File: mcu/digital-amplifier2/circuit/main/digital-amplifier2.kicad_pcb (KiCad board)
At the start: 2 copper layers, 100 x 100 mm, 173 parts, among them J1 USB_B, J2 Barrel_Jack_Switch, J3 AudioJack3_Switch, J4 AudioJack4, J5 ec11, J6 ext_sai, J7 swd, Q1 s8550, SW1 sw1, SW2 sw2, SW3 sw3, T1 Transformer_diy_01, U1 STM32F446RETx, U10 LP2992AIM5-5.0_NOPB, U11 LP2992AIM5-3.3_NOPB, U12 PCM1792A, U13 OPA4134, U2 LP2992AIM5-3.3_NOPB, U3 TPS55340, U4 LP2992AIM5-3.3_NOPB, U5 DLT11H0, U6 SJR-BTM331, U7 TPA6120A2, U8 LT3045xMSE-1, U9 LT3094xMSE, Y1 5032 8m

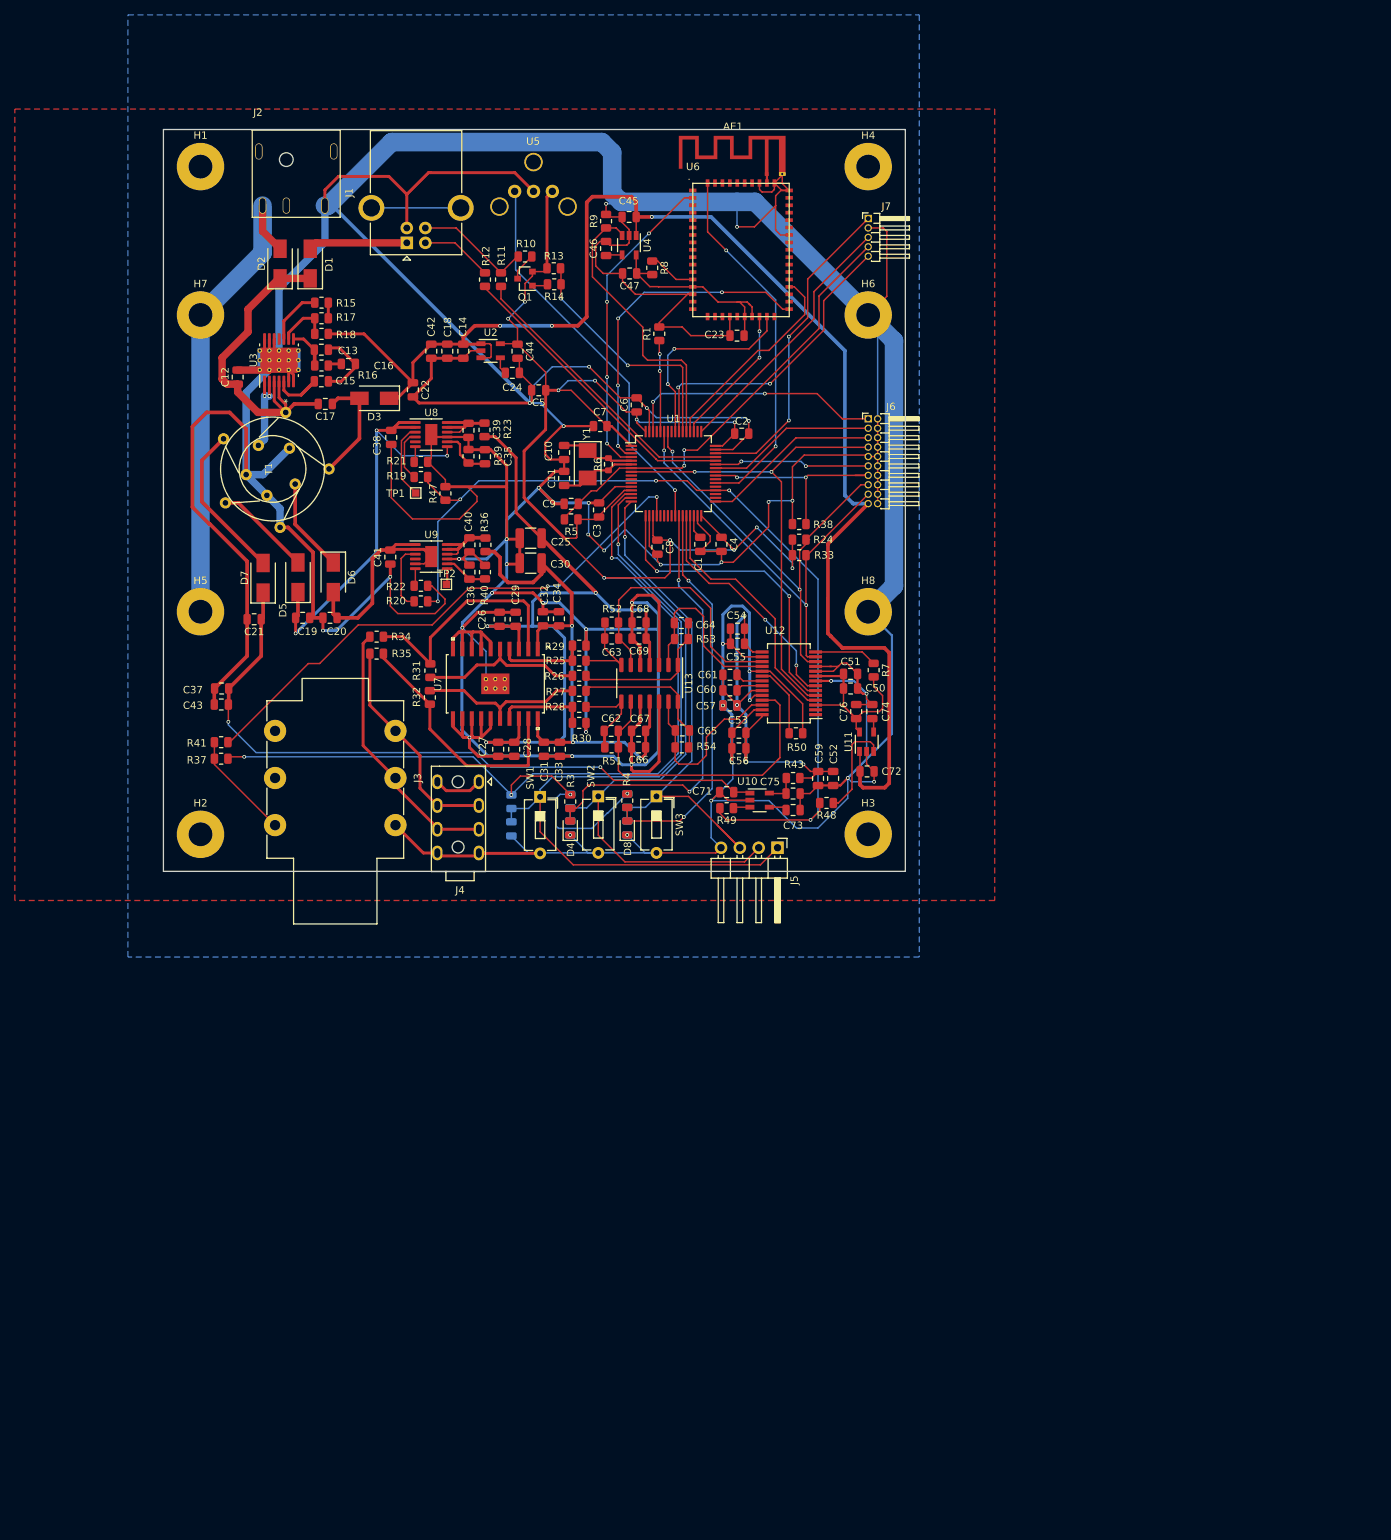
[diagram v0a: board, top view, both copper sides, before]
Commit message: digital-amplifier2_v8
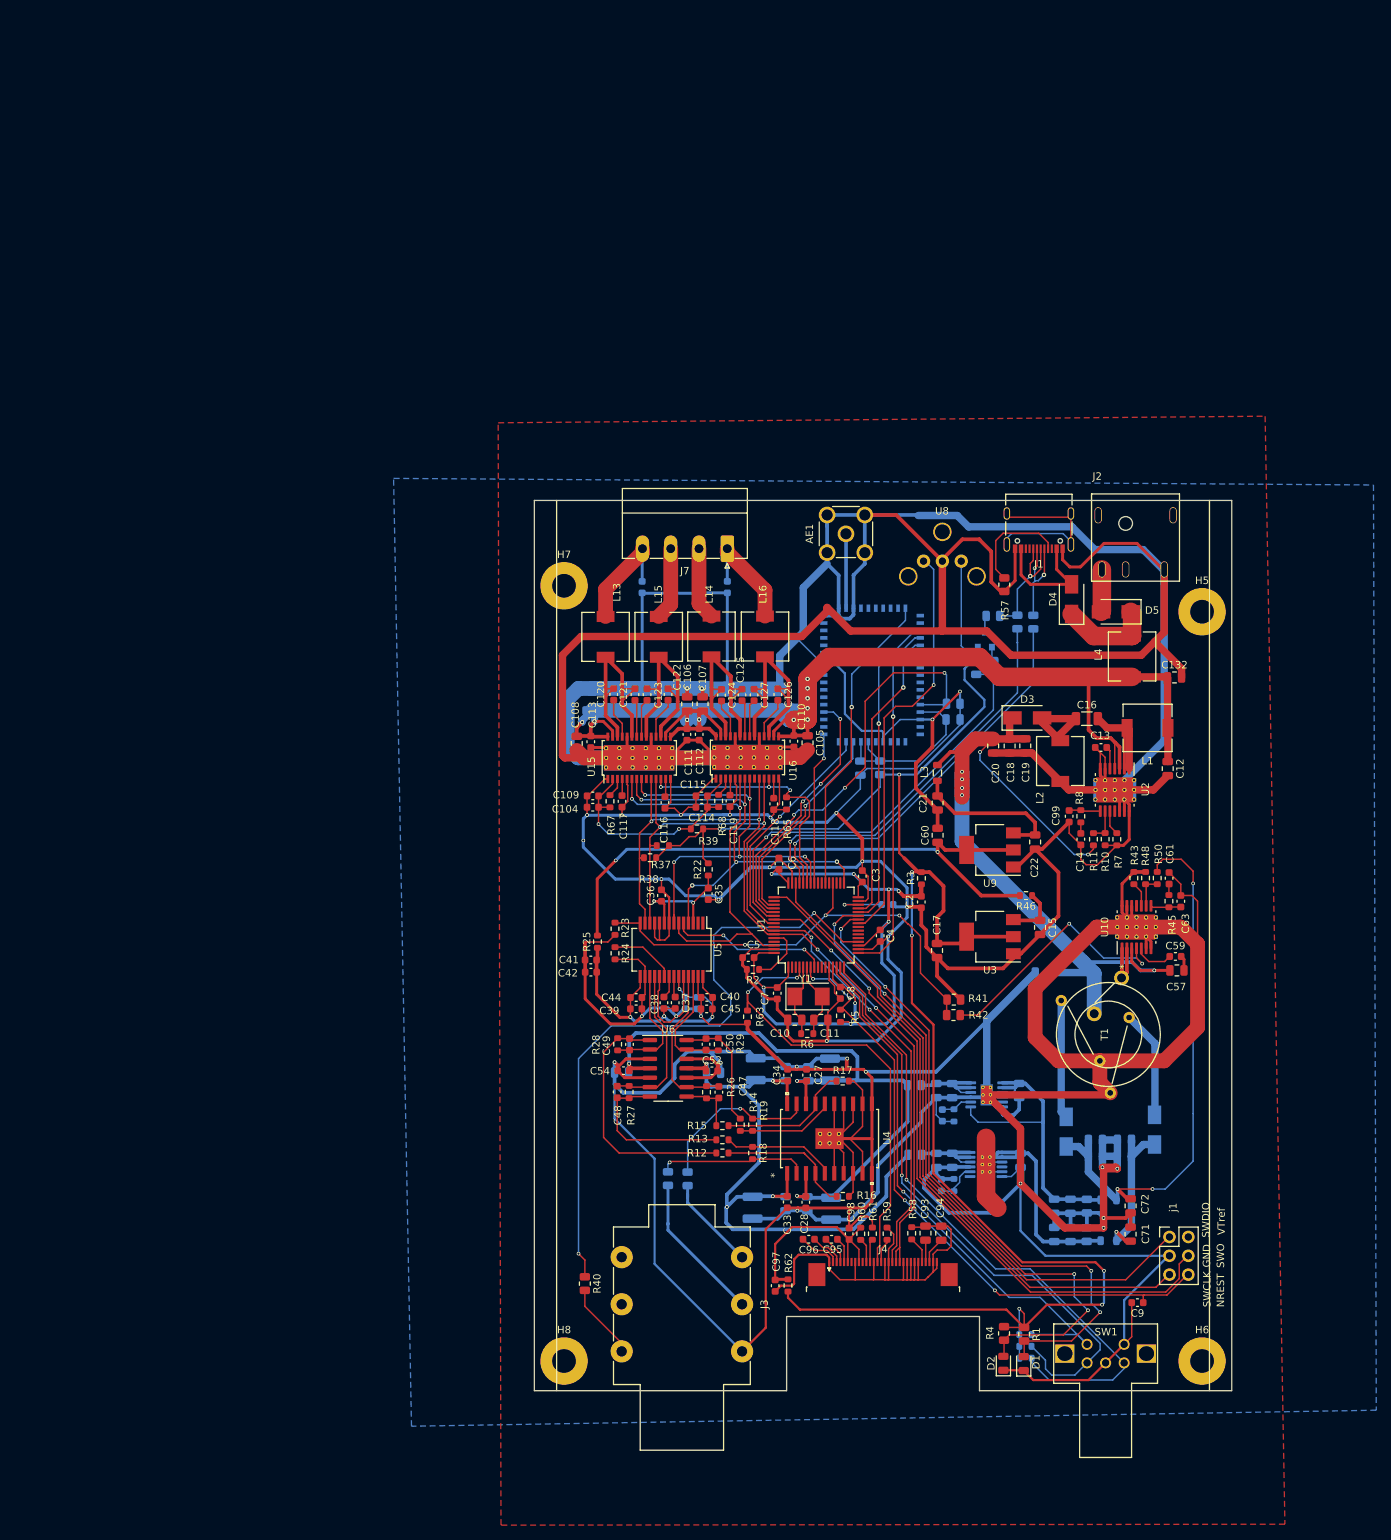
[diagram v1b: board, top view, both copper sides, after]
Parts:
- removed C62, C64, C65: 2.7nf, Capacitor_SMD:C_0805_2012Metric
- removed C66: 10uf, Capacitor_SMD:C_0805_2012Metric
- removed D8: led2, LED_SMD:LED_0805_2012Metric
- removed H1, H2, H3, H4: m3, MountingHole:MountingHole_3.2mm_M3_Pad
- removed J5: ec11, Connector_PinHeader_2.54mm:PinHeader_1x04_P2.54mm_Horizontal
- removed J6: ext_sai, Connector_PinHeader_1.27mm:PinHeader_2x10_P1.27mm_Horizontal
- removed SW2: sw2, Button_Switch_THT:SW_DIP_SPSTx01_Slide_6.7x4.1mm_W7.62mm_P2.54mm_LowProfile
- removed SW3: sw3, Button_Switch_THT:SW_DIP_SPSTx01_Slide_6.7x4.1mm_W7.62mm_P2.54mm_LowProfile
- removed TP1: tp1, TestPoint:TestPoint_Pad_1.0x1.0mm
- removed TP2: tp2, TestPoint:TestPoint_Pad_1.0x1.0mm
- removed U13: OPA4134, Package_SO:SOIC-14_3.9x8.7mm_P1.27mm
- added C100: 100uf, Capacitor_SMD:C_1210_3225Metric, B.Cu at (133.1, 126.9)
- added C101: 100uf, Capacitor_SMD:C_1210_3225Metric, B.Cu at (120.0, 126.8)
- added C102: 100uf, Capacitor_SMD:C_1210_3225Metric, B.Cu at (107.8, 126.8)
- added C103: 100uf, Capacitor_SMD:C_1210_3225Metric, B.Cu at (123.5, 126.8)
- added C104: 4.7uf, Capacitor_SMD:C_0603_1608Metric, F.Cu at (107.9, 141.4)
- added C105: 10uf, Capacitor_SMD:C_0805_2012Metric, F.Cu at (136.8, 132.7)
- added C106: 10uf, Capacitor_SMD:C_0805_2012Metric, F.Cu at (120.6, 127.4)
- added C107: 10uf, Capacitor_SMD:C_0805_2012Metric, F.Cu at (122.7, 127.4)
- added C108: 10uf, Capacitor_SMD:C_0805_2012Metric, F.Cu at (105.7, 132.7)
- added C109: 100nf, Capacitor_SMD:C_0603_1608Metric, F.Cu at (107.9, 139.8)
- added C110: 100nf, Capacitor_SMD:C_0603_1608Metric, F.Cu at (135.0, 132.5)
- added C111: 100nf, Capacitor_SMD:C_0603_1608Metric, F.Cu at (120.6, 131.5)
- added C112: 100nf, Capacitor_SMD:C_0603_1608Metric, F.Cu at (122.2, 131.5)
- added C113: 100nf, Capacitor_SMD:C_0603_1608Metric, F.Cu at (107.6, 132.5)
- added C114: 4.7uf, Capacitor_SMD:C_0603_1608Metric, F.Cu at (122.6, 141.4)
- added C115: 100nf, Capacitor_SMD:C_0603_1608Metric, F.Cu at (122.6, 139.8)
- added C116: 1uf, Capacitor_SMD:C_0603_1608Metric, F.Cu at (117.6, 140.7)
- added C117: 1uf, Capacitor_SMD:C_0603_1608Metric, F.Cu at (111.8, 140.6)
- added C118: 1uf, Capacitor_SMD:C_0603_1608Metric, F.Cu at (132.3, 140.9)
- added C119: 1uf, Capacitor_SMD:C_0603_1608Metric, F.Cu at (126.4, 140.5)
- added C120: 220nf, Capacitor_SMD:C_0603_1608Metric, F.Cu at (110.7, 126.1)
- added C121: 220nf, Capacitor_SMD:C_0603_1608Metric, F.Cu at (113.6, 126.2)
- added C122: 220nf, Capacitor_SMD:C_0603_1608Metric, F.Cu at (118.0, 126.2)
- added C123: 220nf, Capacitor_SMD:C_0603_1608Metric, F.Cu at (115.2, 126.2)
- added C124: 220nf, Capacitor_SMD:C_0603_1608Metric, F.Cu at (125.2, 126.2)
- added C125: 220nf, Capacitor_SMD:C_0603_1608Metric, F.Cu at (128.0, 126.2)
- added C126: 220nf, Capacitor_SMD:C_0603_1608Metric, F.Cu at (132.8, 126.2)
- added C127: 220nf, Capacitor_SMD:C_0603_1608Metric, F.Cu at (129.6, 126.2)
- added C128: 680nf, Capacitor_SMD:C_0603_1608Metric, B.Cu at (114.5, 111.7)
- added C129: 680nf, Capacitor_SMD:C_0603_1608Metric, B.Cu at (122.2, 111.7)
- added C130: 680nf, Capacitor_SMD:C_0603_1608Metric, B.Cu at (118.4, 111.7)
- added C131: 680nf, Capacitor_SMD:C_0603_1608Metric, B.Cu at (126.0, 111.7)
- added C132: 10uf, Capacitor_SMD:C_0805_2012Metric, F.Cu at (186.3, 123.9)
- added C77: 22uf, Capacitor_SMD:C_0805_2012Metric, B.Cu at (165.3, 179.5)
- added C78: 22uf, Capacitor_SMD:C_0805_2012Metric, B.Cu at (165.5, 189.0)
- added C79: 4.7uf, Capacitor_SMD:C_0603_1608Metric, B.Cu at (155.0, 182.9)
- added C80: 4.7uf, Capacitor_SMD:C_0603_1608Metric, B.Cu at (154.9, 192.3)
- added C81: 22uf, Capacitor_SMD:C_0805_2012Metric, B.Cu at (156.3, 179.6)
- added C82: 22uf, Capacitor_SMD:C_0805_2012Metric, B.Cu at (156.3, 188.9)
- added C83: 22uf, Capacitor_SMD:C_0805_2012Metric, B.Cu at (154.2, 179.5)
- added C84: 22uf, Capacitor_SMD:C_0805_2012Metric, B.Cu at (154.2, 189.0)
- added C93: 10uf, Capacitor_SMD:C_0805_2012Metric, F.Cu at (152.7, 198.8)
- added C94: 10uf, Capacitor_SMD:C_0805_2012Metric, F.Cu at (154.8, 198.8)
- added C95: 1uf, Capacitor_SMD:C_0603_1608Metric, F.Cu at (140.1, 199.6)
- added C96: 1uf, Capacitor_SMD:C_0603_1608Metric, F.Cu at (137.0, 199.6)
- added C97: 10uf, Capacitor_SMD:C_0603_1608Metric, F.Cu at (132.5, 205.8)
- added C98: 100nf, Capacitor_SMD:C_0603_1608Metric, F.Cu at (142.4, 198.8)
- added C99: NC, Capacitor_SMD:C_0603_1608Metric, F.Cu at (172.1, 142.6)
- added L1: 22uh / 0630, Inductor_SMD:L_6.3x6.3_H3, F.Cu at (182.7, 130.7)
- added L10: 2.2uh / 0805, Inductor_SMD:L_0805_2012Metric, B.Cu at (177.4, 194.3)
- added L13: 10uh, Inductor_SMD:L_6.3x6.3_H3, F.Cu at (109.6, 118.4)
- added L14: 10uh, Inductor_SMD:L_6.3x6.3_H3, F.Cu at (123.9, 118.3)
- added L15: 10uh, Inductor_SMD:L_6.3x6.3_H3, F.Cu at (116.8, 118.4)
- added L16: 10uh, Inductor_SMD:L_6.3x6.3_H3, F.Cu at (131.1, 118.3)
- added L2: 22uh / 0630, Inductor_SMD:L_6.3x6.3_H3, F.Cu at (170.9, 135.1)
- added L3: 2.2uh / 0805, Inductor_SMD:L_0805_2012Metric, F.Cu at (154.3, 136.7)
- added L4: 4.7uh / 0630, Inductor_SMD:L_6.3x6.3_H3, F.Cu at (180.6, 121.0)
- added L9: 2.2uh / 0805, Inductor_SMD:L_0805_2012Metric, B.Cu at (177.4, 199.8)
- added R2: 9.53kΩ, Resistor_SMD:R_0603_1608Metric, F.Cu at (129.5, 163.2)
- added R45: 2.37k, Resistor_SMD:R_0603_1608Metric, F.Cu at (185.5, 154.0)
- added R55: 10k, Resistor_SMD:R_0603_1608Metric, B.Cu at (166.2, 212.4)
- added R57: 5.1k, Resistor_SMD:R_0805_2012Metric, F.Cu at (163.3, 111.4)
- added R58: 760k, Resistor_SMD:R_0603_1608Metric, F.Cu at (150.9, 198.8)
- added R59: 9.53k, Resistor_SMD:R_0603_1608Metric, F.Cu at (147.5, 198.8)
- added R60: 9.53k, Resistor_SMD:R_0603_1608Metric, F.Cu at (144.0, 198.8)
- added R61: 9.53k, Resistor_SMD:R_0603_1608Metric, F.Cu at (145.6, 198.8)
- added R62: 0Ω, Resistor_SMD:R_0603_1608Metric, F.Cu at (134.2, 205.8)
- added R63: 9.53k, Resistor_SMD:R_0603_1608Metric, F.Cu at (128.7, 169.6)
- added R65: 9.53k, Resistor_SMD:R_0603_1608Metric, F.Cu at (134.0, 140.8)
- added R67: 15k, Resistor_SMD:R_0603_1608Metric, F.Cu at (110.2, 140.5)
- added R68: 47k, Resistor_SMD:R_0603_1608Metric, F.Cu at (124.8, 140.5)
- added U15: tas5805m, Package_SO:HTSSOP-28-1EP_4.4x9.7mm_P0.65mm_EP3.4x9.5mm_ThermalVias, F.Cu at (114.1, 134.7)
- added U16: tas5805m, Package_SO:HTSSOP-28-1EP_4.4x9.7mm_P0.65mm_EP3.4x9.5mm_ThermalVias, F.Cu at (128.7, 134.6)
- added j1: swd_pcb_2.54, misc:swd_pcb_2.54, F.Cu at (191.9, 201.8)
- AE1: footprint RF_Antenna:Texas_SWRA117D_2.4GHz_Left -> Connector_Coaxial:SMA_Molex_73251-2200_Horizontal
- C1: footprint Capacitor_SMD:C_0805_2012Metric -> Capacitor_SMD:C_0603_1608Metric; moved to B.Cu
- C13: value NC -> 47nf; footprint Capacitor_SMD:C_0805_2012Metric -> Capacitor_SMD:C_0603_1608Metric
- C14, C27, C40, C44, C5, C52, C54: value 10uf -> 100nf; footprint Capacitor_SMD:C_0805_2012Metric -> Capacitor_SMD:C_0603_1608Metric
- C15: value 47nf -> 10uf
- C16: value 100nf -> 2.2uf; footprint Capacitor_SMD:C_0805_2012Metric -> Capacitor_SMD:C_1206_3216Metric
- C17: value NC -> 1uf
- C2: value 100nf -> 10uf; footprint Capacitor_SMD:C_0805_2012Metric -> Capacitor_SMD:C_0603_1608Metric
- C20: value 22uf -> 100nf
- C23: value 22uf -> 100uf; footprint Capacitor_SMD:C_0805_2012Metric -> Capacitor_SMD:C_1210_3225Metric; moved to B.Cu
- C24: value 10nf -> 100uf; footprint Capacitor_SMD:C_0805_2012Metric -> Capacitor_SMD:C_1210_3225Metric; moved to B.Cu
- C25: value 100uf -> 10uf; footprint Capacitor_SMD:C_1210_3225Metric -> Capacitor_SMD:C_0805_2012Metric; moved to B.Cu
- C26, C30, C31, C32, C56, D6, D7, Q1: moved to B.Cu
- C28, C3, C33, C34, C39, C4, C45, C6, C8, C9: footprint Capacitor_SMD:C_0805_2012Metric -> Capacitor_SMD:C_0603_1608Metric
- C29: value 100nf -> 100uf; footprint Capacitor_SMD:C_0805_2012Metric -> Capacitor_SMD:C_1210_3225Metric; moved to B.Cu
- C35: value 4.7uf -> 10uf; footprint Capacitor_SMD:C_0805_2012Metric -> Capacitor_SMD:C_0603_1608Metric
- C36: value 4.7uf -> 100nf; footprint Capacitor_SMD:C_0805_2012Metric -> Capacitor_SMD:C_0603_1608Metric
- C37, C38: value 22uf -> 47uf; footprint Capacitor_SMD:C_0805_2012Metric -> Capacitor_SMD:C_0603_1608Metric
- C41: value 22uf -> 10uf; footprint Capacitor_SMD:C_0805_2012Metric -> Capacitor_SMD:C_0603_1608Metric
- C42: value 22uf -> 100nf; footprint Capacitor_SMD:C_0805_2012Metric -> Capacitor_SMD:C_0603_1608Metric
- C43: value 100nf -> 10uf; footprint Capacitor_SMD:C_0805_2012Metric -> Capacitor_SMD:C_0603_1608Metric; moved to B.Cu
- C46: value 10nf -> 100nf; footprint Capacitor_SMD:C_0805_2012Metric -> Capacitor_SMD:C_0603_1608Metric; moved to B.Cu
- C47, C50: value 10uf -> 2.7nf; footprint Capacitor_SMD:C_0805_2012Metric -> Capacitor_SMD:C_0603_1608Metric
- C48, C49: value 10nf -> 2.7nf; footprint Capacitor_SMD:C_0805_2012Metric -> Capacitor_SMD:C_0603_1608Metric; moved to F.Cu
- C51, C53: value 100nf -> 10uf; moved to B.Cu
- C55, C67, C69: value 100nf -> 22uf; moved to B.Cu
- C57: value 100nf -> 10uf
- C59: value 100nf -> 47nf; footprint Capacitor_SMD:C_0805_2012Metric -> Capacitor_SMD:C_0603_1608Metric
- C60: value 47uf -> 1uf
- C61: value 47uf -> 100nf; footprint Capacitor_SMD:C_0805_2012Metric -> Capacitor_SMD:C_0603_1608Metric
- C63: value 2.7nf -> NC; footprint Capacitor_SMD:C_0805_2012Metric -> Capacitor_SMD:C_0603_1608Metric
- C68, C75, C76: value 10uf -> 22uf; moved to B.Cu
- C7: footprint Resistor_SMD:R_0805_2012Metric -> Capacitor_SMD:C_0603_1608Metric
- C70: value 10nf -> 22uf
- C71, C72: value 10uf -> 100nf
- C73, C74: value 10nf -> 22uf; moved to B.Cu
- D1: value ss34 -> led1; footprint Diode_SMD:D_SMA -> LED_SMD:LED_0805_2012Metric
- D2: value ss34 -> led2; footprint Diode_SMD:D_SMA -> LED_SMD:LED_0805_2012Metric
- D4: value led1 -> ss34; footprint LED_SMD:LED_0805_2012Metric -> Diode_SMD:D_SMA
- J1: value USB_B -> USB_C_Receptacle_USB2.0; footprint Connector_USB:USB_B_OST_USB-B1HSxx_Horizontal -> Connector_USB:USB_C_Receptacle_Palconn_UTC16-G
- J4: value AudioJack4 -> 0.96_oled; footprint connector:Jack_3.5mm_4pin -> Connector_FFC-FPC:TE_3-1734839-0_1x30-1MP_P0.5mm_Horizontal
- J7: value swd -> PW_OUT; footprint Connector_PinHeader_1.27mm:PinHeader_1x05_P1.27mm_Horizontal -> Connector_Phoenix_MC:PhoenixContact_MC_1,5_4-G-3.81_1x04_P3.81mm_Horizontal
- R1: value 9.53kΩ -> 9.53k
- R10: value 1.5k -> 1k; footprint Resistor_SMD:R_0805_2012Metric -> Resistor_SMD:R_0603_1608Metric
- R11: value 12Ω -> 5k; footprint Resistor_SMD:R_0805_2012Metric -> Resistor_SMD:R_0603_1608Metric
- R12: value 12Ω -> 1k; footprint Resistor_SMD:R_0805_2012Metric -> Resistor_SMD:R_0603_1608Metric
- R13: value 22k -> 1k; footprint Resistor_SMD:R_0805_2012Metric -> Resistor_SMD:R_0603_1608Metric
- R14: value 5.1k -> 1k; footprint Resistor_SMD:R_0805_2012Metric -> Resistor_SMD:R_0603_1608Metric
- R15: value 80k -> 1k; footprint Resistor_SMD:R_0805_2012Metric -> Resistor_SMD:R_0603_1608Metric
- R16: value 2.37k -> 1k; footprint Resistor_SMD:R_0805_2012Metric -> Resistor_SMD:R_0603_1608Metric
- R17: value 2k -> 1k; footprint Resistor_SMD:R_0805_2012Metric -> Resistor_SMD:R_0603_1608Metric
- R18: value 6.1367k -> 1k; footprint Resistor_SMD:R_0805_2012Metric -> Resistor_SMD:R_0603_1608Metric
- R19: value 1m -> 1k; footprint Resistor_SMD:R_0805_2012Metric -> Resistor_SMD:R_0603_1608Metric
- R20: value 1m -> 39.2Ω; moved to B.Cu
- R21: value 0Ω -> 39.2Ω; moved to B.Cu
- R22, R26, R27, R28, R29, R5: footprint Resistor_SMD:R_0805_2012Metric -> Resistor_SMD:R_0603_1608Metric
- R23: value 0Ω -> 9.53k; footprint Resistor_SMD:R_0805_2012Metric -> Resistor_SMD:R_0603_1608Metric
- R24: value 4.7k -> 10k; footprint Resistor_SMD:R_0805_2012Metric -> Resistor_SMD:R_0603_1608Metric
- R25: value 1k -> 0Ω; footprint Resistor_SMD:R_0805_2012Metric -> Resistor_SMD:R_0603_1608Metric
- R3: value 9.53k -> 0Ω; footprint Resistor_SMD:R_0805_2012Metric -> Resistor_SMD:R_0603_1608Metric
- R30: value 1k -> 9.53k; moved to B.Cu
- R31: value 1k -> 0; moved to B.Cu
- R32: value 1k -> 1.5k; moved to B.Cu
- R33: value 4.7k -> 12Ω; moved to B.Cu
- R34: value 39.2Ω -> 12Ω; moved to B.Cu
- R35: value 39.2Ω -> 22k; moved to B.Cu
- R36: value 0Ω -> 5.1k; moved to B.Cu
- R37, R38: value 9.53k -> 4.7k; footprint Resistor_SMD:R_0805_2012Metric -> Resistor_SMD:R_0603_1608Metric
- R39: value 150k -> 0Ω; footprint Resistor_SMD:R_0805_2012Metric -> Resistor_SMD:R_0603_1608Metric
- R40: value 150k -> 9.53k
- R42: moved to F.Cu
- R43: value 0Ω -> 43k; footprint Resistor_SMD:R_0805_2012Metric -> Resistor_SMD:R_0603_1608Metric
- R44: value 9.53k -> 10k
- R46: value 9.53k -> 0Ω; footprint Resistor_SMD:R_0805_2012Metric -> Resistor_SMD:R_0603_1608Metric; moved to F.Cu
- R47, R49: value 9.53k -> 10k; footprint Resistor_SMD:R_0805_2012Metric -> Resistor_SMD:R_0603_1608Metric; moved to B.Cu
- R48: value 9.53k -> 1k; footprint Resistor_SMD:R_0805_2012Metric -> Resistor_SMD:R_0603_1608Metric
- R50: value 10k -> 13k; footprint Resistor_SMD:R_0805_2012Metric -> Resistor_SMD:R_0603_1608Metric
- R51, R52: value 1k -> 150k; footprint Resistor_SMD:R_0805_2012Metric -> Resistor_SMD:R_0603_1608Metric; moved to B.Cu
- R53, R54: value 1k -> 0Ω; moved to B.Cu
- R7: value 9.53k -> 43k; footprint Resistor_SMD:R_0805_2012Metric -> Resistor_SMD:R_0603_1608Metric
- R8: value 9.53k -> 2.37k; footprint Resistor_SMD:R_0805_2012Metric -> Resistor_SMD:R_0603_1608Metric
- R9: value 9.53k -> 10k; moved to B.Cu
- SW1: value sw1 -> ec11; footprint Button_Switch_THT:SW_DIP_SPSTx01_Slide_6.7x4.1mm_W7.62mm_P2.54mm_LowProfile -> misc:ec11_horizontal
- T1: value Transformer_diy_01 -> Transformer_1P_2S; footprint misc:Transformer_diy_01 -> misc:Transformer_diy_02
- U10: value LP2992AIM5-5.0_NOPB -> TPS55340; footprint Package_TO_SOT_SMD:TSOT-23-5 -> Package_SO:HTSSOP-14-1EP_4.4x5mm_P0.65mm_EP3.4x5mm_Mask3x3.1mm_ThermalVias
- U11: value LP2992AIM5-3.3_NOPB -> LT3045xMSE-1; footprint Package_TO_SOT_SMD:TSOT-23-5 -> Package_SO:MSOP-12-1EP_3x4mm_P0.65mm_EP1.65x2.85mm_ThermalVias; moved to B.Cu
- U12: value PCM1792A -> LT3094xMSE; footprint Package_SO:SSOP-28_5.3x10.2mm_P0.65mm -> Package_SO:MSOP-12-1EP_3x4mm_P0.65mm_EP1.65x2.85mm_ThermalVias; moved to B.Cu
- U2: value LP2992AIM5-3.3_NOPB -> TPS55340; footprint Package_TO_SOT_SMD:TSOT-23-5 -> Package_SO:HTSSOP-14-1EP_4.4x5mm_P0.65mm_EP3.4x5mm_Mask3x3.1mm_ThermalVias
- U3: value TPS55340 -> AMS1117-3.3; footprint Package_SO:HTSSOP-14-1EP_4.4x5mm_P0.65mm_EP3.4x5mm_Mask3x3.1mm_ThermalVias -> Package_TO_SOT_SMD:SOT-223-3_TabPin2
- U4: value LP2992AIM5-3.3_NOPB -> TPA6120A2; footprint Package_TO_SOT_SMD:TSOT-23-5 -> ti:TPA6120A2DWP
- U5: value DLT11H0 -> PCM1792A; footprint connector:spdif-DLT11H0 -> Package_SO:SSOP-28_5.3x10.2mm_P0.65mm
- U6: value SJR-BTM331 -> OPA4134; footprint misc:SJR-BTM331 -> Package_SO:SOIC-14_3.9x8.7mm_P1.27mm
- U7: value TPA6120A2 -> SJR-BTM331; footprint ti:TPA6120A2DWP -> misc:SJR-BTM331; moved to B.Cu
- U8: value LT3045xMSE-1 -> DLT11H0; footprint Package_SO:MSOP-12-1EP_3x4mm_P0.65mm_EP1.65x2.85mm -> connector:spdif-DLT11H0
- U9: value LT3094xMSE -> AMS1117-5.0; footprint Package_SO:MSOP-12-1EP_3x4mm_P0.65mm_EP1.65x2.85mm -> Package_TO_SOT_SMD:SOT-223-3_TabPin2
- moved D2 177.4 mm to (163.2, 216.3)
- moved D1 176.7 mm to (166.0, 216.3)
- moved R9 151.2 mm to (174.4, 199.0)
- moved H6 148.0 mm to (190.0, 216.0)
- moved R1 143.5 mm to (166.0, 212.4), turned to 270 degrees
- moved R47 139.0 mm to (166.2, 214.0), turned to 0 degrees
- moved T1 136.0 mm to (177.4, 172.0)
- moved C12 136.0 mm to (185.4, 136.1), turned to 270 degrees
- moved H5 135.0 mm to (190.0, 115.0)
- moved D6 133.4 mm to (183.6, 184.8)
- moved R16 132.2 mm to (141.6, 193.8)
- moved C9 132.0 mm to (181.3, 208.1)
- moved D7 131.5 mm to (171.7, 185.1)
- moved R18 124.8 mm to (129.4, 188.0), turned to 270 degrees
- moved R17 124.5 mm to (141.6, 178.3)
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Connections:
- C12 pad 1: /power/vcc1 -> VCC
- C14 pad 1: +5V -> Net-(C14-Pad1)
- C16 pad 2: GND -> Net-(C16-Pad2)
- C17 pad 1: /power/t1a -> +3V3
- C17 pad 2: /power/vcc1 -> GND
- C18 pad 1: +5V -> +7.5V
- C19 pad 1: +15V -> +7.5V
- C2 pad 1: +3V3 -> /stm32/vdd1
- C20 pad 1: GND -> +7.5V
- C20 pad 2: -15V -> GND
- C21 pad 1: +7.5V -> Net-(C21-Pad1)
- C22 pad 1: +5V -> Net-(C21-Pad1)
- C23 pad 1: /Bluetooth/vdd_x -> +12V
- C24 pad 1: Net-(C24-Pad1) -> +12V
- C29 pad 1: +12V -> -12V
- C3 pad 1: +3V3 -> /stm32/vdd1
- C35 pad 1: Net-(C35-Pad1) -> +3.3VDAC
- C36 pad 1: GND -> +3.3VDAC
- C36 pad 2: Net-(C36-Pad2) -> GND
- C37 pad 1: +7.5V -> Net-(C37-Pad1)
- C37 pad 2: GND -> /PCM1792/vdd2
- C38 pad 1: +15V -> Net-(C38-Pad1)
- C38 pad 2: GND -> /PCM1792/vdd2
- C39 pad 1: Net-(C39-Pad1) -> /PCM1792/vdd2
- C4 pad 1: +3V3 -> /stm32/vdd1
- C40 pad 1: GND -> /PCM1792/vdd2
- C40 pad 2: Net-(C40-Pad2) -> GND
- C41 pad 1: GND -> /PCM1792/vdd2
- C41 pad 2: -15V -> GND
- C42 pad 1: +5V -> /PCM1792/vdd2
- C43 pad 1: +7.5V -> /PCM1792/vdd2
- C44 pad 1: +3V3 -> /PCM1792/vdd2
- C45 pad 1: +5V -> /PCM1792/vdd2
- C46 pad 1: Net-(C46-Pad1) -> /PCM1792/vdd2
- C47 pad 1: /Bluetooth/vdd_x -> /OPA4134/OUTC
- C47 pad 2: GND -> /OPA4134/INC
- C48 pad 1: /ec11_sw -> /TPA6120A2/LIN-
- C48 pad 2: GND -> /OPA4134/INB
- C49 pad 1: /ec11_a -> /TPA6120A2/LIN+
- C49 pad 2: GND -> /OPA4134/INA
- C5 pad 1: +3V3 -> /stm32/vdd1
- C50 pad 1: +3.3VDAC -> /OPA4134/OUTD
- C50 pad 2: GND -> /OPA4134/IND
- C51 pad 1: +3.3VDAC -> -12V
- C52 pad 1: /PCM1792/vdd2 -> -12V
- C53 pad 1: /PCM1792/vdd2 -> +12V
- C54 pad 1: /PCM1792/vdd2 -> +12V
- C55 pad 1: /PCM1792/vdd2 -> /Bluetooth/vdd_x
- C56 pad 1: /PCM1792/vdd2 -> /Bluetooth/vdd_x
- C57 pad 1: /PCM1792/vdd2 -> +7.5V
- C58 pad 1: /PCM1792/vdd2 -> +7.5V
- C59 pad 1: /PCM1792/vdd2 -> Net-(C59-Pad1)
- C6 pad 1: +3V3 -> /stm32/vdd1
- C60 pad 1: Net-(C60-Pad1) -> +5V
- C60 pad 2: /PCM1792/vdd2 -> GND
- C61 pad 2: /PCM1792/vdd2 -> GND
- C63 pad 1: /TPA6120A2/LIN+ -> Net-(C63-Pad1)
- C63 pad 2: /OPA4134/INA -> GND
- C67 pad 1: -12V -> Net-(C67-Pad1)
- C68 pad 1: +12V -> /hp_power/FB1
- C69 pad 1: +12V -> Net-(C67-Pad1)
- C7 pad 1: +3V3 -> /stm32/vdd1
- C70 pad 1: /ec11_b -> /hp_power/FB1
- C71 pad 1: +7.5V -> Net-(C67-Pad1)
- C72 pad 1: +5V -> /hp_power/FB1
- C73 pad 1: Net-(C73-Pad1) -> -15V
- C74 pad 1: Net-(C74-Pad1) -> +15V
- C75 pad 1: +5VA -> -15V
- C76 pad 1: +3.3VDAC -> +15V
- C8 pad 1: +3V3 -> /stm32/vdd1
- D1 pad 1: /power/vcc1 -> GND
- D1 pad 2: VBUS -> /stm32/led1
- D2 pad 1: /power/vcc1 -> GND
- D2 pad 2: VCC -> /stm32/led2
- D3 pad 1: +5V -> +7.5V
- D3 pad 2: /power/t1a -> Net-(C16-Pad1)
- D4 pad 1: GND -> /connector/vcc1
- D4 pad 2: /stm32/led1 -> Net-(D4-Pad2)
- D5 pad 1: +15V -> /connector/vcc1
- D5 pad 2: /power/t2a -> Net-(D5-Pad2)
- D6 pad 1: /power/t2c -> /hp_power/out-
- D6 pad 2: -15V -> Net-(C67-Pad1)
- D7 pad 1: +7.5V -> /hp_power/FB1
- D7 pad 2: /power/t3a -> /hp_power/out+
- H5 pad 1: VCC -> (no net)
- H6 pad 1: GND -> (no net)
- H7 pad 1: VCC -> (no net)
- H8 pad 1: GND -> (no net)
- J2 pad 1: VCC -> Net-(D5-Pad2)
- J7 pad 1: /swdio -> /out_b-
- J7 pad 2: GND -> /out_b+
- J7 pad 3: /swclk -> /out_a-
- J7 pad 4: /nrst -> /out_a+
- R1 pad 1: /stm32/BOOT -> +3V3
- R1 pad 2: GND -> /stm32/led1
- R10 pad 1: Net-(Q1-Pad3) -> Net-(R10-Pad1)
- R10 pad 2: Net-(J1-Pad3) -> GND
- R11 pad 1: /USB_DP -> +7.5V
- R11 pad 2: Net-(J1-Pad3) -> Net-(R10-Pad1)
- R12 pad 1: /USB_DM -> Net-(R12-Pad1)
- R12 pad 2: Net-(J1-Pad2) -> /TPA6120A2/LIN+
- R13 pad 1: +3V3 -> Net-(R13-Pad1)
- R13 pad 2: /USB_CO -> /TPA6120A2/LIN-
- R14 pad 1: /USB_CO -> Net-(R14-Pad1)
- R14 pad 2: Net-(Q1-Pad1) -> /OPA4134/OUTD
- R15 pad 2: GND -> /OPA4134/OUTC
- R16 pad 1: Net-(C13-Pad1) -> Net-(R12-Pad1)
- R16 pad 2: Net-(C16-Pad1) -> GND
- R17 pad 1: Net-(R17-Pad1) -> Net-(R15-Pad1)
- R18 pad 1: +5V -> Net-(R13-Pad1)
- R18 pad 2: Net-(R17-Pad1) -> Net-(R18-Pad2)
- R19 pad 1: /hp_power/on1 -> Net-(R14-Pad1)
- R19 pad 2: /hp_en -> Net-(R19-Pad2)
- R20 pad 1: /hp_power/on2 -> /ROUT
- R20 pad 2: /hp_en -> Net-(R18-Pad2)
- R21 pad 1: Net-(R21-Pad1) -> /LOUT
- R21 pad 2: GND -> Net-(R19-Pad2)
- R22 pad 1: GND -> +3.3VDAC
- R22 pad 2: Net-(R22-Pad2) -> +3V3
- R23 pad 1: +12V -> GND
- R23 pad 2: Net-(C39-Pad1) -> /hp_en
- R24 pad 1: +3V3 -> Net-(R24-Pad1)
- R24 pad 2: /I2C_SCL -> GND
- R25 pad 1: Net-(R25-Pad1) -> /PCM1792/vdd2
- R25 pad 2: /TPA6120A2/LIN+ -> +5V
- R26 pad 1: Net-(R26-Pad1) -> /OPA4134/OUTC
- R26 pad 2: /TPA6120A2/LIN- -> /OPA4134/INC
- R27 pad 1: Net-(R27-Pad1) -> /TPA6120A2/LIN-
- R27 pad 2: /OPA4134/OUTD -> /OPA4134/INB
- R28 pad 1: Net-(R28-Pad1) -> /TPA6120A2/LIN+
- R28 pad 2: /OPA4134/OUTC -> /OPA4134/INA
- R29 pad 1: Net-(R25-Pad1) -> /OPA4134/OUTD
- R29 pad 2: GND -> /OPA4134/IND
- R3 pad 1: +3V3 -> /stm32/vdd1
- R3 pad 2: /stm32/led1 -> +3V3
- R30 pad 1: Net-(R28-Pad1) -> /BT_en
- R31 pad 1: Net-(R26-Pad1) -> /Bluetooth/vdd_x
- R31 pad 2: Net-(R31-Pad2) -> +3V3
- R32 pad 1: Net-(R27-Pad1) -> Net-(Q1-Pad3)
- R32 pad 2: Net-(R32-Pad2) -> /connector/d+
- R33 pad 1: +3V3 -> /USB_DP
- R33 pad 2: /I2C_SDA -> /connector/d+
- R34 pad 1: /ROUT -> /USB_DM
- R34 pad 2: Net-(R31-Pad2) -> Net-(J1-PadA7)
- R35 pad 1: /LOUT -> +3V3
- R35 pad 2: Net-(R32-Pad2) -> /USB_EN
- R36 pad 1: -12V -> /USB_EN
- R36 pad 2: Net-(C40-Pad2) -> Net-(Q1-Pad1)
- R37 pad 1: Net-(J3-PadSN) -> +3V3
- R37 pad 2: +3V3 -> /I2C_SCL
- R38 pad 1: GND -> +3V3
- R38 pad 2: /ext_irq -> /I2C_SDA
- R39 pad 1: Net-(C35-Pad1) -> /TAS5805M/dvdd1
- R39 pad 2: GND -> +3V3
- R40 pad 1: GND -> /jack_in
- R40 pad 2: Net-(C36-Pad2) -> Net-(J3-PadSN)
- R41 pad 1: /jack_in -> /hp_en
- R41 pad 2: Net-(J3-PadSN) -> GND
- R42 pad 1: +3V3 -> /hp_power/enx
- R42 pad 2: /ec11_sw -> /hp_en
- R43 pad 1: /PCM1792/vdd2 -> Net-(R43-Pad1)
- R43 pad 2: +5VA -> GND
- R44 pad 1: +3V3 -> +15V
- R44 pad 2: /ec11_a -> GND
- R46 pad 1: +3V3 -> Net-(C15-Pad1)
- R46 pad 2: /ec11_b -> +5V
- R47 pad 1: /hp_en -> +3V3
- R47 pad 2: GND -> /ec11_a
- R48 pad 1: /hp_power/on3 -> Net-(R48-Pad1)
- R48 pad 2: /hp_en -> GND
- R49 pad 1: /hp_power/on4 -> +3V3
- R49 pad 2: /hp_en -> /ec11_b
- R5 pad 1: +3V3 -> /stm32/vdd1
- R50 pad 1: Net-(R50-Pad1) -> /hp_power/FB1
- R50 pad 2: GND -> Net-(R48-Pad1)
- R51 pad 1: /OPA4134/OUTC -> Net-(C79-Pad1)
- R51 pad 2: /OPA4134/INC -> GND
- R52 pad 1: /TPA6120A2/LIN+ -> GND
- R52 pad 2: /OPA4134/INA -> Net-(C80-Pad2)
- R53 pad 1: /TPA6120A2/LIN- -> +12V
- R53 pad 2: /OPA4134/INB -> Net-(C81-Pad1)
- R54 pad 1: /OPA4134/OUTD -> -12V
- R54 pad 2: /OPA4134/IND -> Net-(C82-Pad2)
- R7 pad 2: +3.3VDAC -> GND
- R8 pad 1: Net-(R8-Pad1) -> Net-(C99-Pad1)
- R8 pad 2: /Bluetooth/vdd_x -> Net-(C14-Pad1)
- R9 pad 1: /BT_en -> -15V
- T1 pad 1: /power/vcc1 -> +7.5V
- T1 pad 2: /power/SW -> Net-(T1-Pad2)
- T1 pad 3: /power/t1a -> /hp_power/out-
- T1 pad 5: /power/t2a -> GND
- T1 pad 6: GND -> /hp_power/out+
- U1 pad 1: +3V3 -> /stm32/vdd1
- U1 pad 13: +3V3 -> /stm32/vdd1
- U1 pad 19: +3V3 -> /stm32/vdd1
- U1 pad 3: /BT_connected -> (no net)
- U1 pad 32: +3V3 -> /stm32/vdd1
- U1 pad 4: /BT_music -> /oled_en
- U1 pad 40: /ext_irq -> (no net)
- U1 pad 41: (no net) -> /BT_connected
- U1 pad 43: /ext_en -> /5805_en
- U1 pad 48: +3V3 -> /stm32/vdd1
- U1 pad 54: /USB_CO -> /USB_EN
- U1 pad 64: +3V3 -> /stm32/vdd1
- U10 pad 1: +7.5V -> Net-(T1-Pad2)
- U10 pad 2: GND -> Net-(T1-Pad2)
- U10 pad 3: /hp_power/on4 -> +7.5V
- U10 pad 4: Net-(C73-Pad1) -> /hp_power/enx
- U10 pad 5: +5VA -> Net-(C59-Pad1)
- U11 pad 1: +5V -> +15V
- U11 pad 2: GND -> +15V
- U11 pad 3: /hp_power/on3 -> (no net)
- U11 pad 4: Net-(C74-Pad1) -> +15V
- U11 pad 5: +3.3VDAC -> (no net)
- U12 pad 1: (no net) -> -15V
- U12 pad 10: GND -> Net-(C82-Pad2)
- U12 pad 11: GND -> Net-(C82-Pad2)
- U12 pad 12: /I2C_SCL -> Net-(C82-Pad2)
- U12 pad 13: /I2C_SDA -> -15V
- U12 pad 2: (no net) -> -15V
- U12 pad 3: +3.3VDAC -> -15V
- U12 pad 4: /SAI_SCK_A -> (no net)
- U12 pad 5: /SAI_MCK -> -15V
- U12 pad 6: /SAI_FS_A -> GND
- U12 pad 7: /SAI_SD_A -> (no net)
- U12 pad 8: GND -> Net-(C80-Pad2)
- U12 pad 9: +3.3VDAC -> GND
- U2 pad 1: +5V -> Net-(C16-Pad2)
- U2 pad 2: GND -> Net-(C16-Pad2)
- U2 pad 3: +5V -> VCC
- U2 pad 4: Net-(C24-Pad1) -> VCC
- U2 pad 5: +3V3 -> Net-(C13-Pad1)
- U3 pad 1: /power/SW -> GND
- U3 pad 2: /power/SW -> +3V3
- U3 pad 3: /power/vcc1 -> Net-(C15-Pad1)
- U4 pad 1: +5V -> -12V
- U4 pad 2: GND -> Net-(R18-Pad2)
- U4 pad 3: /BT_en -> +12V
- U4 pad 4: Net-(C46-Pad1) -> Net-(R12-Pad1)
- U4 pad 5: /Bluetooth/vdd_x -> Net-(R13-Pad1)
- U5 pad 1: /SPDIF_RX -> (no net)
- U5 pad 2: GND -> (no net)
- U5 pad 3: +3V3 -> +3.3VDAC
- U6 pad 1: (no net) -> /TPA6120A2/LIN+
- U6 pad 10: (no net) -> GND
- U6 pad 11: (no net) -> -12V
- U6 pad 12: (no net) -> GND
- U6 pad 13: Net-(R8-Pad1) -> /OPA4134/IND
- U6 pad 14: /Bluetooth/vdd_x -> /OPA4134/OUTD
- U6 pad 2: /BT_music -> /OPA4134/INA
- U6 pad 3: (no net) -> GND
- U6 pad 4: (no net) -> +12V
- U6 pad 5: (no net) -> GND
- U6 pad 6: (no net) -> /OPA4134/INB
- U6 pad 7: (no net) -> /TPA6120A2/LIN-
- U6 pad 8: (no net) -> /OPA4134/OUTC
- U6 pad 9: (no net) -> /OPA4134/INC
- U7 pad 1: -12V -> (no net)
- U7 pad 10: GND -> (no net)
- U7 pad 11: GND -> (no net)
- U7 pad 12: GND -> (no net)
- U7 pad 13: GND -> /BT_en
- U7 pad 14: GND -> /Bluetooth/vdd_x
- U7 pad 16: Net-(R27-Pad1) -> (no net)
- U7 pad 17: Net-(R28-Pad1) -> (no net)
- U7 pad 18: +12V -> (no net)
- U7 pad 19: Net-(R32-Pad2) -> (no net)
- U7 pad 2: Net-(R31-Pad2) -> (no net)
- U7 pad 20: -12V -> (no net)
- U7 pad 3: +12V -> /SAI_SD_A
- U7 pad 4: Net-(R25-Pad1) -> /SAI_FS_A
- U7 pad 5: Net-(R26-Pad1) -> /SAI_SCK_A
- U7 pad 6: GND -> (no net)
- U7 pad 7: GND -> (no net)
- U7 pad 8: GND -> (no net)
- U7 pad 9: GND -> (no net)
- U8 pad 1: +15V -> /SPDIF_RX
- U8 pad 2: +15V -> GND
- U8 pad 3: Net-(TP1-Pad1) -> +3V3
- U9 pad 1: -15V -> GND
- U9 pad 2: -15V -> +5V
- U9 pad 3: /hp_power/on2 -> Net-(C21-Pad1)
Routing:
- net GND: track 1343.5 -> 1754.1 mm, vias 41 -> 32
- net VCC: track 65.0 -> 210.8 mm, vias 0 -> 10
- net +5V: track 213.9 -> 80.8 mm, vias 3 -> 2
- net /stm32/vdd1: track 0.00 -> 107.9 mm, vias 0 -> 8
- net /hp_power/FB1: track 0.00 -> 78.5 mm, vias 0 -> 3
- net /hp_en: track 126.4 -> 62.8 mm, vias 5 -> 3
- net /oled_en: track 0.00 -> 63.5 mm, vias 0 -> 2
- net /I2C_SDA: track 58.0 -> 116.9 mm, vias 2 -> 4
- net /USB_EN: track 0.00 -> 58.0 mm, vias 0 -> 1
- net /I2C_SCL: track 58.9 -> 114.6 mm, vias 2 -> 4
- net /swclk: track 35.5 -> 87.4 mm
- net /swo_tdo: track 41.3 -> 91.1 mm
- net /power/vcc1: track 46.2 -> 0.00 mm
- net +3V3: track 301.2 -> 255.1 mm, vias 15 -> 7
- net /SAI_MCK: track 66.5 -> 21.3 mm
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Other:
- board size 100 x 100 mm -> 94 x 120 mm
